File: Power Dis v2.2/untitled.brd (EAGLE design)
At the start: 83.8 x 115 mm, 77 parts, among them J1 PCIE-098-02-X-D-TH, Q1 MMBT2222, U1 MCP9808MSOP, U2 ADS1115IDGST

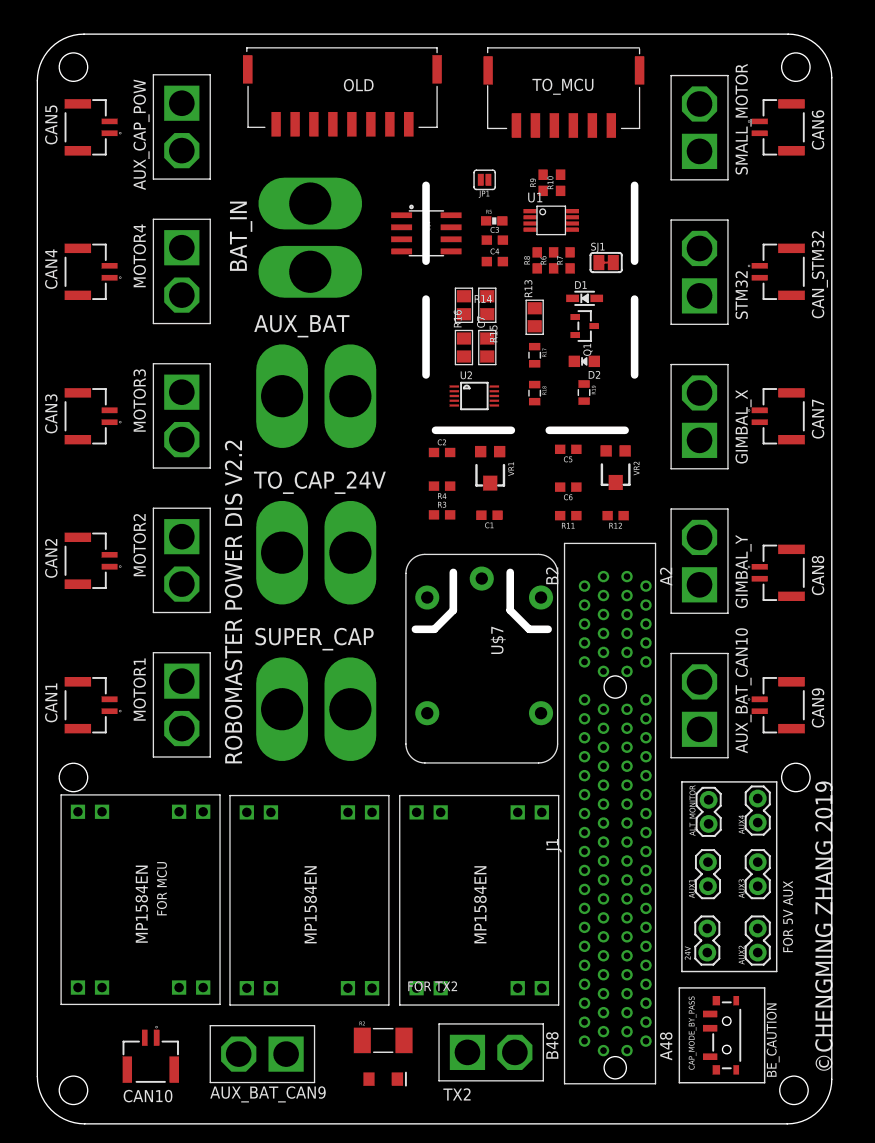
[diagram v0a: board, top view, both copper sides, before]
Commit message: shit
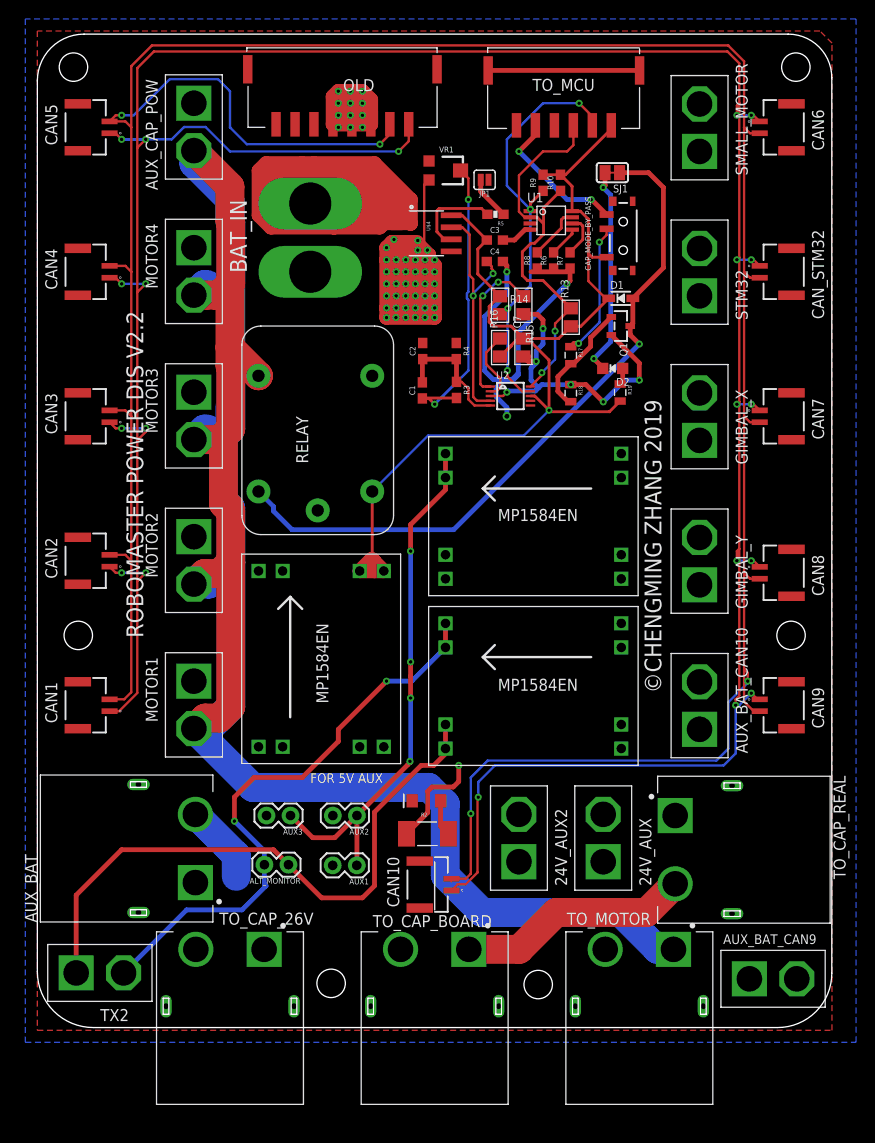
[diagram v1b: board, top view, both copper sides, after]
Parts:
- removed 24V, AUX4: (no value), SparkFun-Connectors:1X02
- removed C5, C6: 0.1uF, SparkFun-Capacitors:0603
- removed J1: PCIE-098-02-X-D-TH, PCIE-098-02-X-D-TH:PCIE-098-02-X-D-TH
- removed R11: 10k, SparkFun-Resistors:0603
- removed R12: 2.0k, SparkFun-Resistors:0603
- removed SUPER_CAP, TO_CAP_24V: XT60, NewKevinMade:XT60
- removed U$7: RELAY_G5LE, microbuilder:RELAY_G5LE-1
- removed VR2: 10k, SparkFun-Resistors:TRIMPOT-SMD-TC33X
- added 24V_AUX, 24V_AUX2: XT30, NewKevinMade:XT30
- added RELAY: RELAY_G5LE, microbuilder:RELAY_G5LE-1
- added TO_CAP_26V, TO_CAP_BOARD, TO_CAP_REAL, TO_MOTOR: XT60PW-M, XT60PW-M:AMASS_XT60PW-M
- AUX_BAT: value XT60 -> XT60PW-M; device NewKevinMade:XT60 -> XT60PW-M:AMASS_XT60PW-M
- moved CAP_MODE_BY_PASS 85.0 mm to (61.8, 59.7)
- moved U$5 60.5 mm to (63.4, 38.5), turned to 180 degrees
- moved AUX3 49.8 mm to (26.7, -1.48), turned to 180 degrees
- moved U$2 49.6 mm to (63.4, 20.6), turned to 180 degrees
- moved AUX_BAT_CAN9 49.5 mm to (75.1, -18.7), turned to 0 degrees
- moved AUX_BAT 46.3 mm to (10.7, -4.95), turned to 90 degrees
- moved AUX2 44.7 mm to (33.7, -1.48), turned to 180 degrees
- moved ALT_MONITOR 44.5 mm to (26.5, -6.66), turned to 180 degrees
- moved TX2 42.1 mm to (4.09, -18.1)
- moved AUX1 37.1 mm to (33.7, -6.73), turned to 180 degrees
- moved CAN10 35.6 mm to (43.7, -8.76), turned to 270 degrees
- moved VR1 31.8 mm to (43.1, 66.6), turned to 270 degrees
- moved U$1 31.8 mm to (38.3, 4.00)
- moved BAT_STATUS 29.7 mm to (41.0, 0.07), turned to 180 degrees
- moved R2 22.3 mm to (41.1, -3.40), turned to 180 degrees
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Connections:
- net CANH renamed CAN_H
- net CANL renamed CAN_L
- net CHARGE_OR_NOT renamed AUX_DIGI
- removed net CAP_ANALOG_OUT: C5.2, C6.1, R11.1, R12.2, U2.6
- removed net N$10: J1.A7, J1.A8
- removed net N$11: J1.A10, J1.A11, J1.A9
- removed net N$16: J1.A12, J1.A13, J1.A14, J1.A15, J1.A16, J1.A17, J1.A18, J1.A19, J1.A20, J1.A21, J1.A22
- removed net N$18: J1.A35, J1.A36, J1.A37, J1.A38, J1.A39, J1.A40, J1.A41, J1.A42, J1.A43, J1.A44, J1.A45, J1.A46, J1.A47, J1.A48, J1.A49
- removed net N$19: J1.A23, J1.A24, J1.A25, J1.A26, J1.A27, J1.A28, J1.A29, J1.A30, J1.A31, J1.A32, J1.A33, J1.A34
- removed net N$2: J1.A1, J1.A2
- removed net N$3: J1.A3, J1.A4
- removed net N$6: C5.1, R11.2, VR2.2
- removed net N$9: J1.A5, J1.A6
- new net CAP_MOTOR_24V: AUX_CAP_POW.P$2, MOTOR1.P$2, MOTOR2.P$2, MOTOR3.P$2, MOTOR4.P$2, RELAY.4, TO_MOTOR.1
- net 5V_AUX: no longer AUX4.1
- net BAT_24V: now also 24V_AUX.P$2, 24V_AUX2.P$2, AUX_BAT.2, RELAY.1, RELAY.3, TO_CAP_26V.1; no longer 24V.2, AUX_BAT.1, TO_CAP_24V.1, U$7.1, U$7.3
- net BAT_GND: now also 24V_AUX.P$1, 24V_AUX2.P$1, AUX_BAT.1, TO_CAP_26V.2, TO_CAP_BOARD.2, TO_CAP_REAL.1, TO_MOTOR.2; no longer 24V.1, AUX4.2, AUX_BAT.2, C6.2, R12.1, SUPER_CAP.2, TO_CAP_24V.2, VR2.1
- net CAP_24V: now also TO_CAP_BOARD.1, TO_CAP_REAL.2; no longer AUX_CAP_POW.P$2, MOTOR1.P$2, MOTOR2.P$2, MOTOR3.P$2, MOTOR4.P$2, SUPER_CAP.1, U$7.4, VR2.3
- net MCU_VCC: now also RELAY.2; no longer U$7.2
- net N$12: now also RELAY.5; no longer U$7.5
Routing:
- net CAN_L: track 0.00 -> 322.3 mm, vias 0 -> 20
- net CAN_H: track 0.00 -> 310.8 mm, vias 0 -> 4
- net CAP_MOTOR_24V: track 0.00 -> 231.6 mm
- net BAT_IN: track 0.00 -> 142.5 mm
- net BAT_24V: track 0.00 -> 121.0 mm, vias 0 -> 54
- net MCU_VCC: track 0.00 -> 117.4 mm, vias 0 -> 1
- net N$12: track 0.00 -> 73.9 mm, vias 0 -> 1
- net ALT_GND: track 0.00 -> 65.2 mm
- net ALT_VCC: track 0.00 -> 61.7 mm, vias 0 -> 2
- net 5V_AUX: track 0.00 -> 56.4 mm, vias 0 -> 4
- net SDA: track 0.00 -> 46.0 mm, vias 0 -> 4
- net BAT_GND: track 0.00 -> 44.4 mm, vias 0 -> 3
- net SCL: track 0.00 -> 43.5 mm, vias 0 -> 2
- net GND: track 0.00 -> 36.4 mm, vias 0 -> 6
- net N$8: track 0.00 -> 31.8 mm, vias 0 -> 2
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- added copper zone on layer 16, net BAT_24V
- added copper zone on layer 1, net BAT_GND
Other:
- board size 83.8 x 115 mm -> 83.8 x 104.8 mm
- board text removed: "BE_CAUTION"
- board text removed: "FOR MCU"
- board text removed: "FOR TX2"
